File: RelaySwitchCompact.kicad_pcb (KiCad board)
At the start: 2 copper layers, 34 x 17 mm, 13 parts, among them J1 Conn_01x05_Pin, K1 1-1721150-0, U1 FOD817ASD, U2 FMMT634QTA

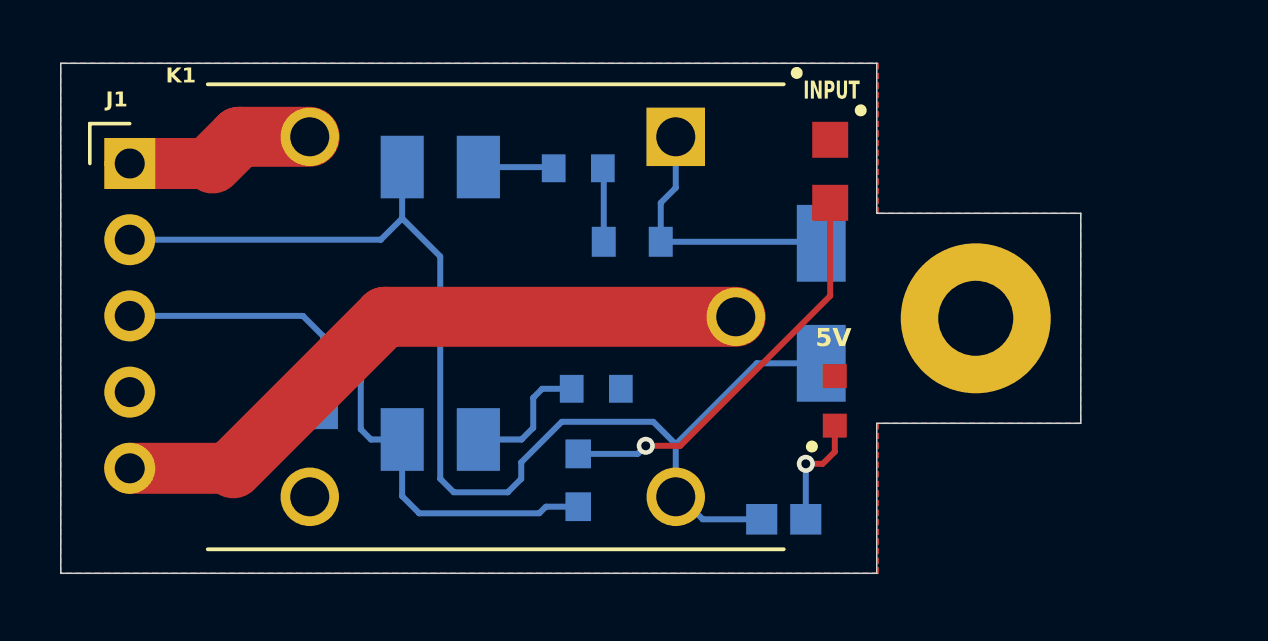
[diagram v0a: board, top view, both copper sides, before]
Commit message: updated and cleaned up files.
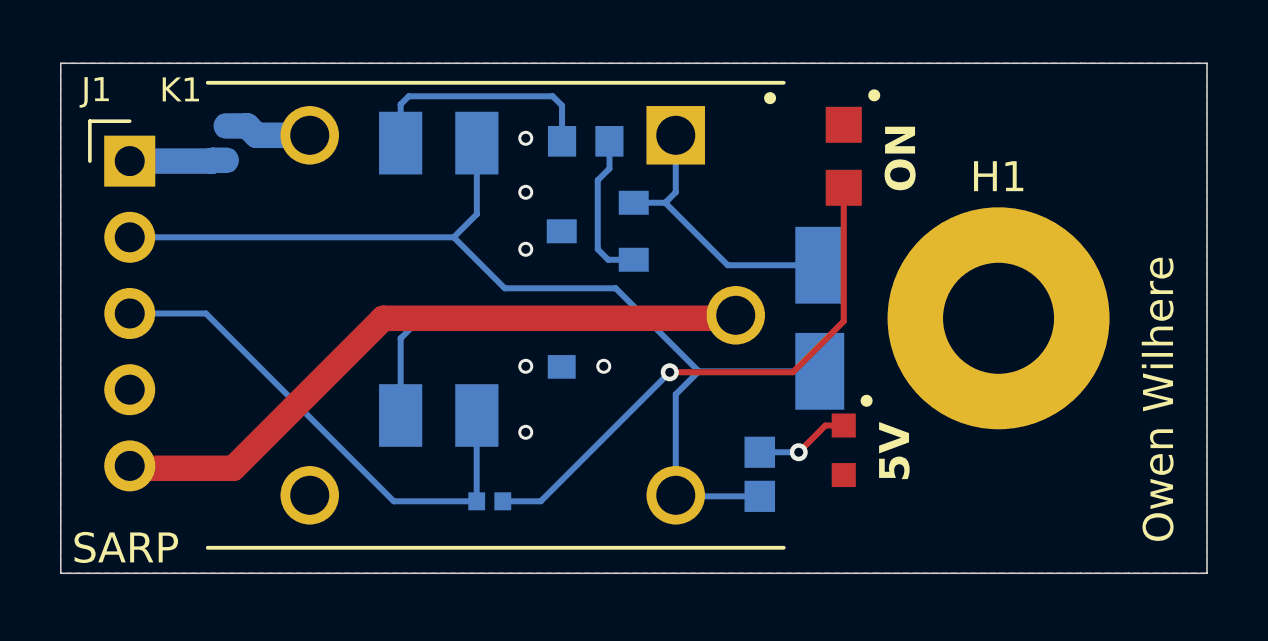
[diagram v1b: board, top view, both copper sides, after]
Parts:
- removed Mount: MountingHole_2.5mm_Pad, MountingHole:MountingHole_2.5mm_Pad
- removed REF**: RC0603N_PAN, footprints68R:RC0603N_PAN-M
- added F1: Fuse, Diode_SMD:D_0402_1005Metric_Pad0.77x0.64mm_HandSolder, B.Cu at (155.5, 97.7)
- added H1: MountingHole_Pad, MountingHole:MountingHole_3.7mm_Pad, F.Cu at (181.3, 103.5)
- D1, R3, U1, U2: moved to B.Cu
- J1: value Conn_01x05_Pin -> 350-10-105-00-001101
- R1: value 330R -> 140; moved to B.Cu
- R2: value 100R -> 1k; footprint AC0603JR-07100RL:RESC1608X55N -> RG1608N-102-D-T5:RESC1608X50N; moved to B.Cu
- R4: value 10k -> 68R; footprint CRCW060310K0DHEAP:RESC1508X50N -> CRCW0402140RFKEDC:RESC1005X35N; moved to B.Cu
- moved R4 6.62 mm to (164.3, 109.6), turned to 180 degrees
- moved U2 1.93 mm to (167.9, 100.6), turned to 180 degrees
- moved R3 1.93 mm to (166.7, 104.3), turned to 90 degrees
- moved R1 1.70 mm to (173.3, 108.7), turned to -90 degrees
- moved LED1 1.68 mm to (176.1, 107.9), turned to -90 degrees
- moved R2 0.93 mm to (167.5, 97.6)
- moved U1 0.80 mm to (162.6, 102.2)
- moved LED2 0.67 mm to (176.1, 98.1)
- moved D1 0.50 mm to (175.3, 103.5)
- moved J1 0.08 mm to (152.3, 98.3)
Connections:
- net /+5V renamed +5V
- J1 pad 4: /GND -> GND
- K1 pad 4: /GND -> GND
- K1 pad 5: /RelayIn -> Net-(F1-Pad1)
- LED1 pad 1: /GND -> GND
- LED2 pad C: /GND -> GND
- R3 pad 1: /GND -> GND
- R4 pad 1: /GND -> Net-(LED2-PadA)
- U2 pad 3: /GND -> GND
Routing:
- net Net-(R2-Pad1): track 2.53 -> 8.10 mm
- net +5V: track 40.8 -> 35.7 mm
- net Net-(LED2-PadA): track 13.7 -> 18.3 mm
- net Net-(R3-Pad2): track 4.40 -> 8.30 mm
- net Net-(F1-Pad1): track 0.00 -> 3.60 mm
- net GND: track 0.00 -> 3.51 mm, vias 0 -> 6
- net /GPIO: track 20.5 -> 17.0 mm
- net /RelayIn: track 6.37 -> 3.23 mm
- net Net-(U2-B): track 2.46 -> 5.11 mm
- net Net-(LED1-A): track 3.86 -> 3.17 mm
- added copper zone on B.Cu, net GND
- added copper zone on F.Cu, net GND
- removed copper zone on B.Cu, net /GND
- removed copper zone on F.Cu, net /GND
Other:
- board size 34 x 17 mm -> 38.2 x 17 mm
- board text added: "ON"
- board text added: "Owen Wilhere"
- board text added: "SARP"
- board text removed: "D1"
- board text removed: "INPUT"
- board text removed: "J1"
- board text removed: "K1"
- board text removed: "R1"
- board text removed: "R2"
- board text removed: "R3"
- board text removed: "R4"
- board text removed: "R5"
- board text removed: "U1"
- board text removed: "U2"
